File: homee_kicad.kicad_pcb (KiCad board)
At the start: 2 copper layers, 114 x 85 mm, 22 parts, among them J1 Screw_Terminal_01x02, J2 476421001, J3 Screw_Terminal_01x02, K1 ORWH-SH-105D1F,000, Q1 2N7002, U1 ESP-01v090, U2 LD1117S33TR_SOT223, U4 PC817

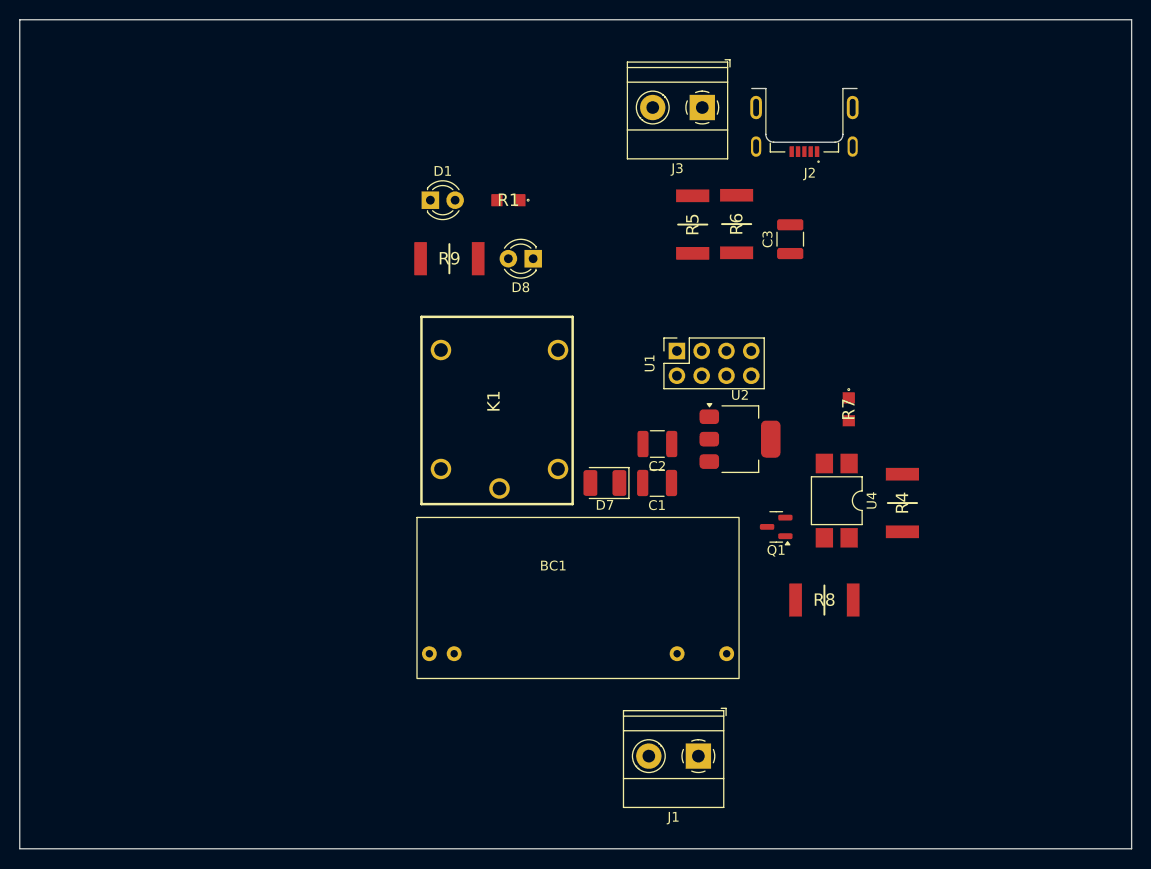
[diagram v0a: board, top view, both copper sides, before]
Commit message: Test W/O routes
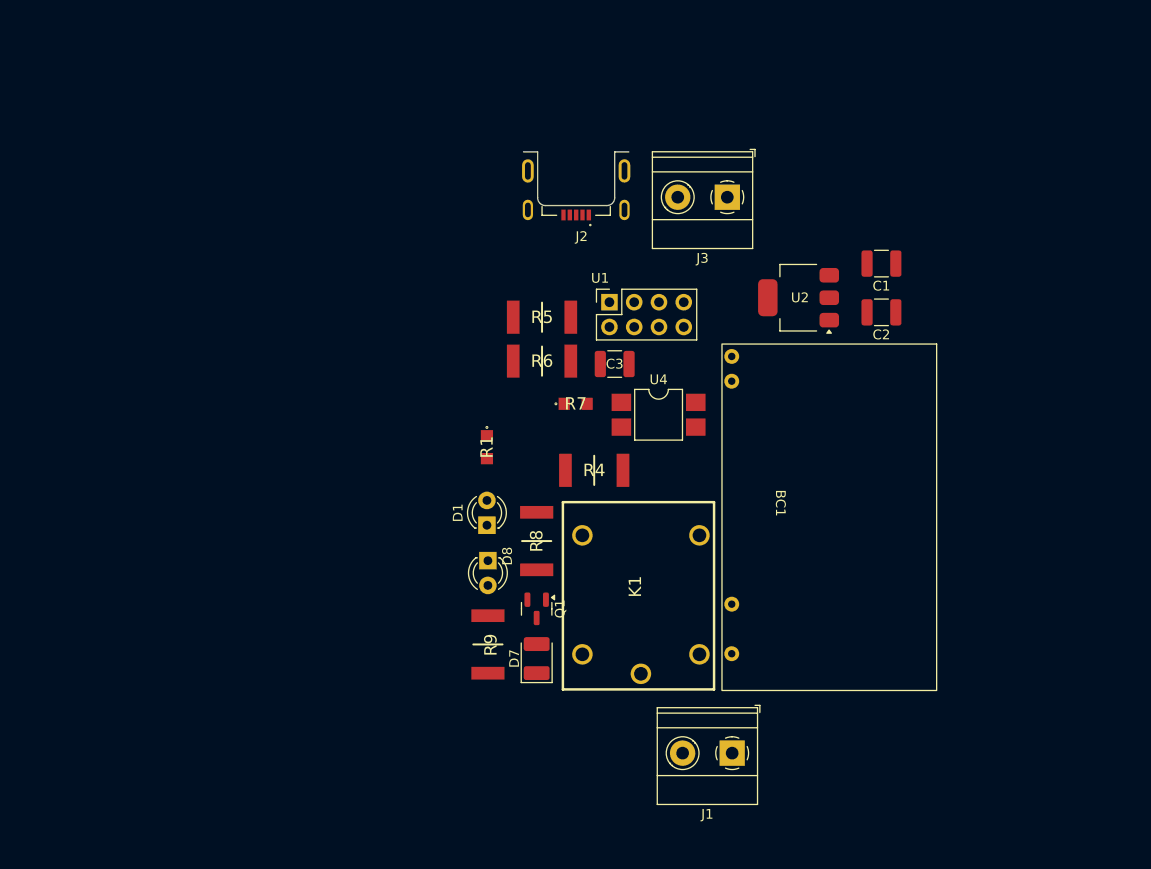
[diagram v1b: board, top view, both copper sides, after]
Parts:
- BC1: footprint Connect:Buck Connect -> Homme:Buck Connect
- moved R9 39.7 mm to (209.0, 144.1), turned to -90 degrees
- moved D1 33.8 mm to (208.9, 131.8), turned to 90 degrees
- moved C1 32.2 mm to (249.3, 105.0)
- moved R4 31.8 mm to (219.9, 126.2), turned to 0 degrees
- moved D8 31.3 mm to (209.0, 135.5), turned to -90 degrees
- moved R8 30.1 mm to (214.0, 133.4), turned to -90 degrees
- moved R7 28.0 mm to (218.0, 119.4), turned to 0 degrees
- moved C2 26.6 mm to (249.3, 110.0)
- moved Q1 26.0 mm to (214.0, 140.4), turned to -90 degrees
- moved R1 25.4 mm to (208.9, 123.8), turned to -90 degrees
- moved R6 24.4 mm to (214.6, 115.0), turned to 0 degrees
- moved J2 24.3 mm to (218.1, 96.7)
- moved K1 23.9 mm to (232.2, 129.5)
- moved BC1 23.2 mm to (233.0, 129.6), turned to -90 degrees
- moved C3 22.1 mm to (222.0, 115.3), turned to 0 degrees
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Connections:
- net /5V renamed +5V
- net /VCC renamed VCC
- BC1 pad 4: /GND -> GND
- C1 pad 1: /GND -> GND
- C2 pad 1: /GND -> GND
- C3 pad 2: /GND -> GND
- D1 pad 1: /GND -> GND
- J2 pad 5: /GND -> GND
- Q1 pad 2: Net-(D7-A) -> GND
- Q1 pad 3: /GND -> Net-(D7-A)
- R8 pad 1: /GND -> GND
- U1 pad 2: /GND -> GND
- U2 pad 1: /GND -> GND
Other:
- board size 114 x 85 mm -> 10.8 x 5.5 mm
